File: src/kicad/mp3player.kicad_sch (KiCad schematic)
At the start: 0 parts

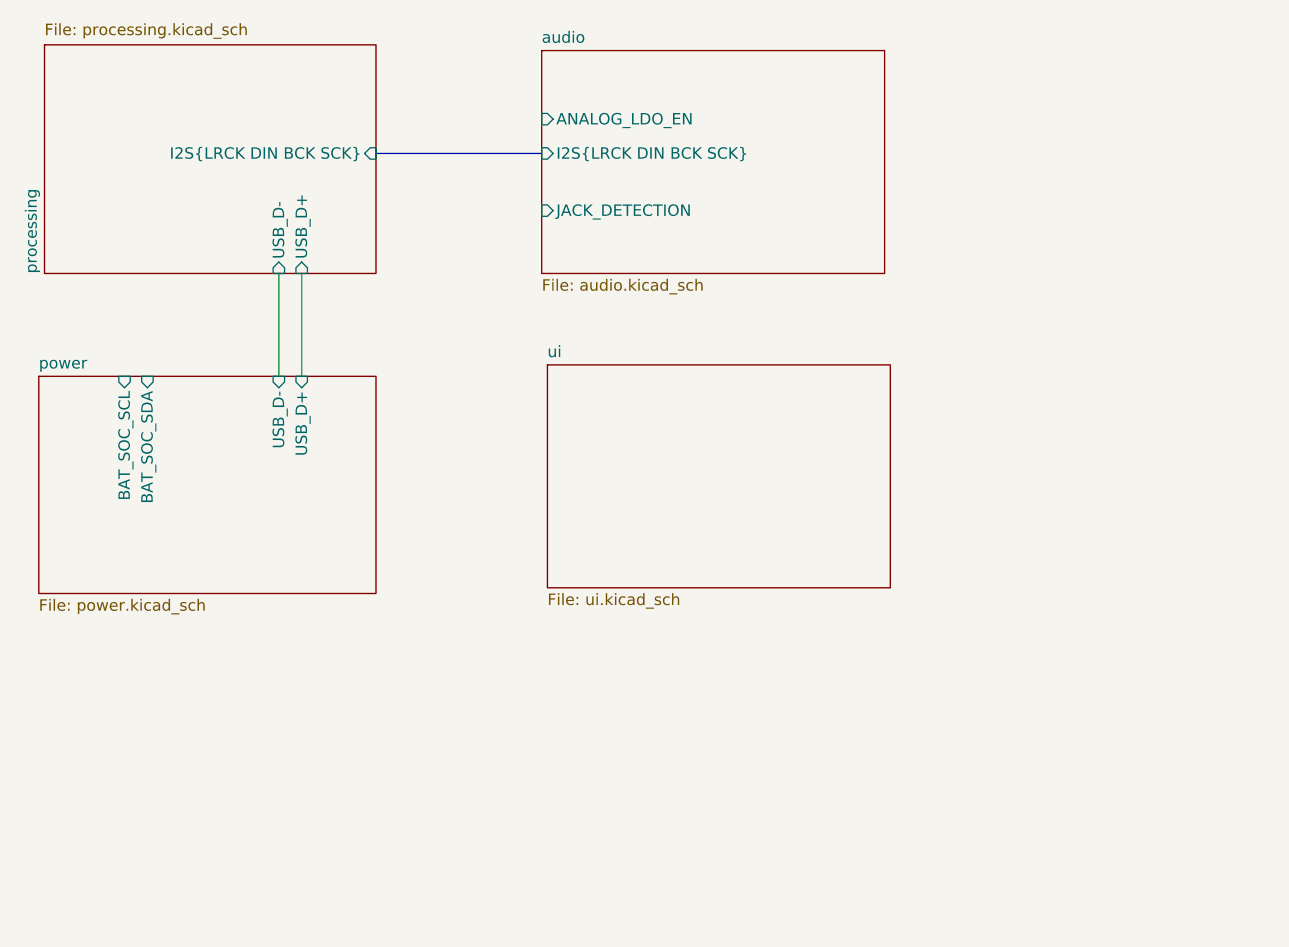
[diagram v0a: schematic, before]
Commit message: progress + new journal entry!
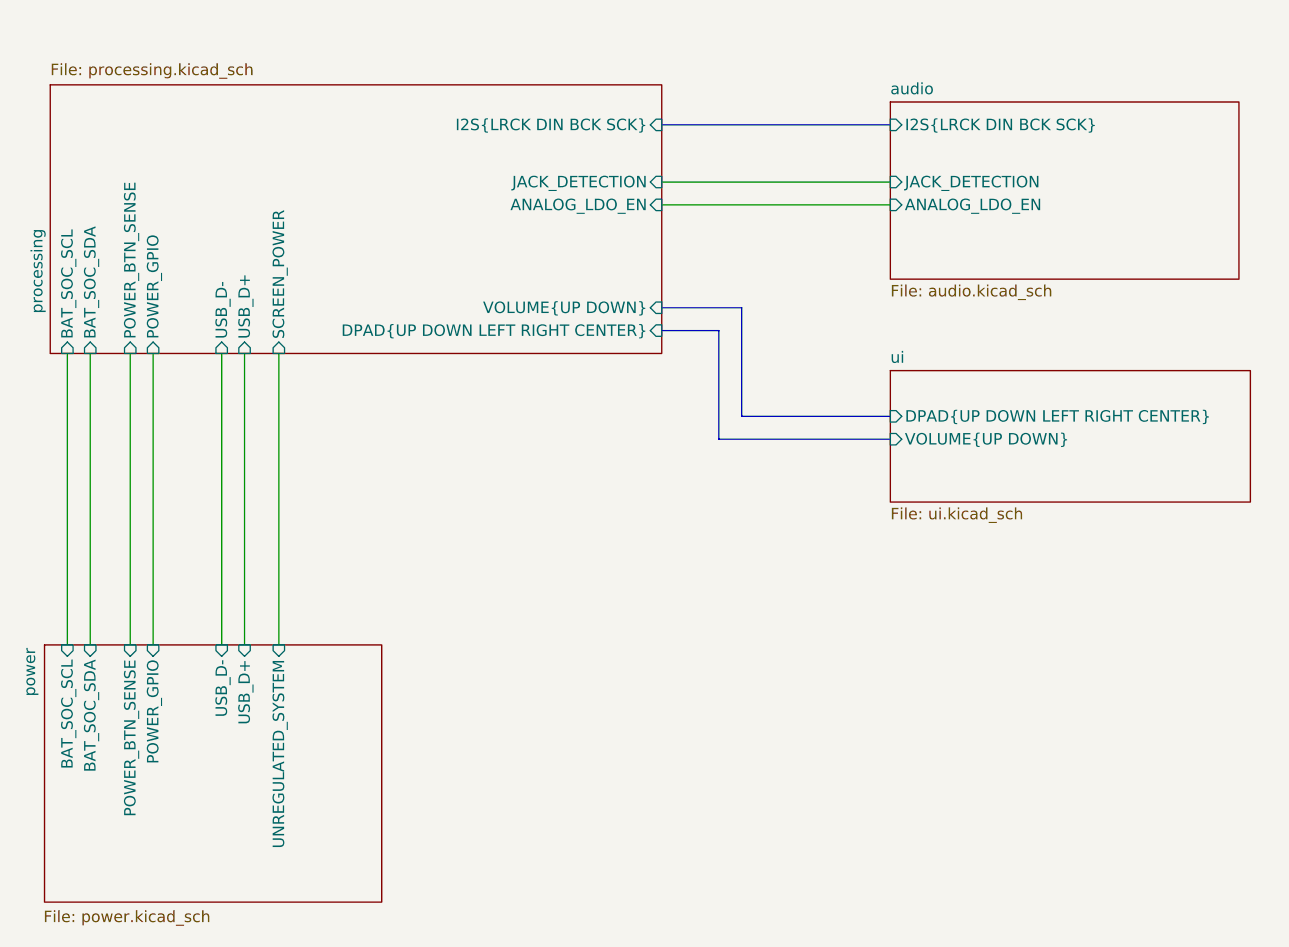
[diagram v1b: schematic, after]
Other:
- sheet power ports: added POWER_BTN_SENSE, POWER_GPIO, UNREGULATED_SYSTEM; removed none
- sheet processing ports: added ANALOG_LDO_EN, BAT_SOC_SCL, BAT_SOC_SDA, DPAD{UP DOWN LEFT RIGHT CENTER}, JACK_DETECTION, POWER_BTN_SENSE, POWER_GPIO, SCREEN_POWER, VOLUME{UP DOWN}; removed none
- sheet ui ports: added DPAD{UP DOWN LEFT RIGHT CENTER}, VOLUME{UP DOWN}; removed none
